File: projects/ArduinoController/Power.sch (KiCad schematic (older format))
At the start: 22 parts, among them CN1 DCBARREL, CON1 USB-MICRO, IC2 OPAMP-DUALU, IC3 OPAMP-LM358, Q3 MOSFET-P, Q4 MOSFET-P, U4 NCP1117, U5 MCP1700, U6 ISL21070

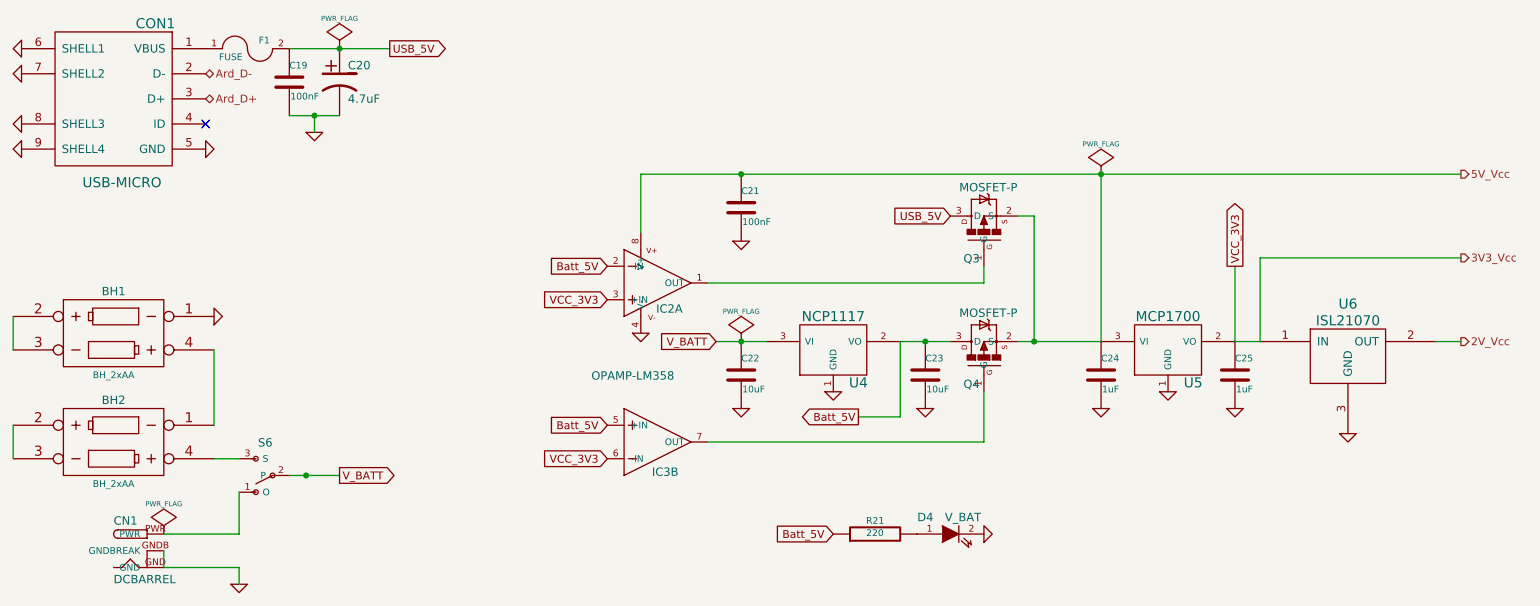
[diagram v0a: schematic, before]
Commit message: footprints done
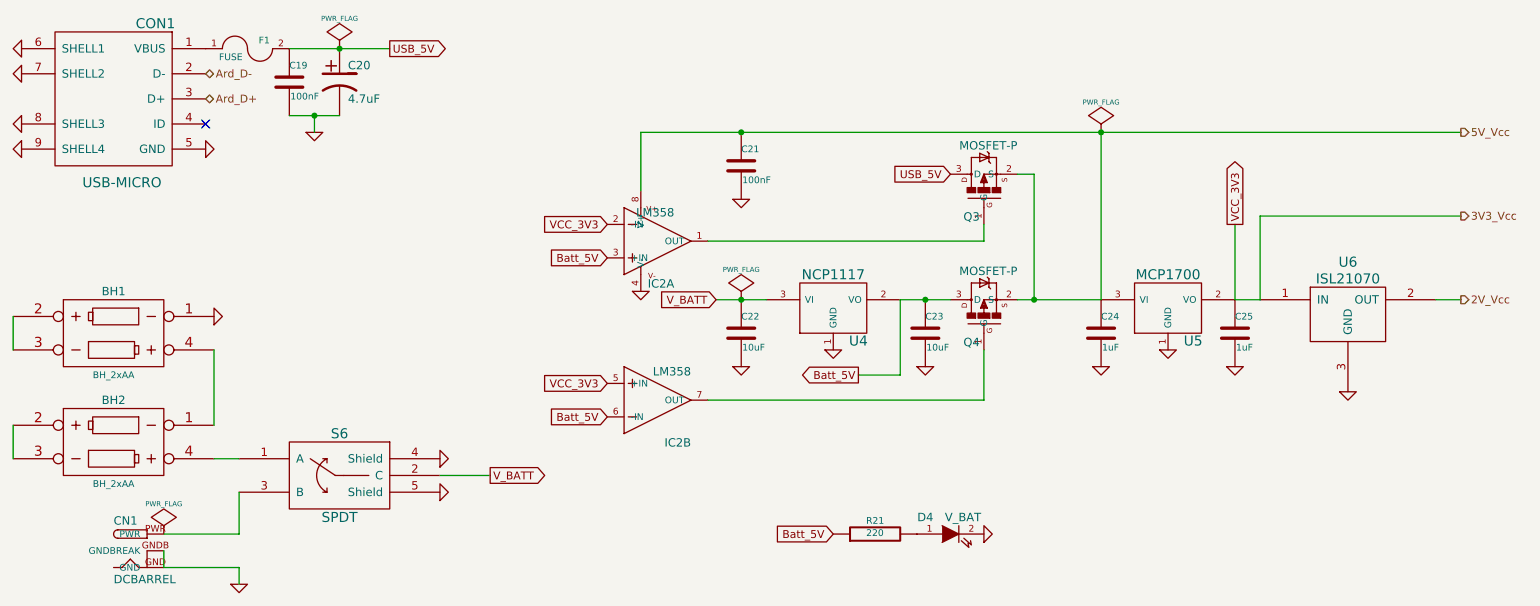
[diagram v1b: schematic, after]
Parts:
- removed IC3: OPAMP-LM358, SparkFun-SO08, symbol OPAMP-DUALU
- removed S6: SWITCH-SPSTPTH2, switch, symbol SWITCH-SPSTPTH2
- added unit 2 of IC2
- added S6: SPDT, symbol SPDT
- IC2: value OPAMP-DUALU -> LM358
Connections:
- net Batt_5V: now also IC2.3 (+IN), IC2.6 (-IN); no longer IC2.2 (-IN)
- net GND: now also S6.4 (Shield), S6.5 (Shield)
- net VCC_3V3: now also IC2.2 (-IN), IC2.5 (+IN); no longer IC2.3 (+IN)
- net V_BATT: now also S6.2 (C)
- net at Q4.1 (G): now also IC2.7 (OUT)
- net at CN1.PWR: now also S6.3 (B)
- net at BH2.4: now also S6.1 (A)
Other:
- moved on the sheet: C21, C22, C23, C24, C25, Q3, Q4, U4, U5, U6
